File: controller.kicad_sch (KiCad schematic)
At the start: 6 parts, among them U1 ESP32-C6-DevKitC-1

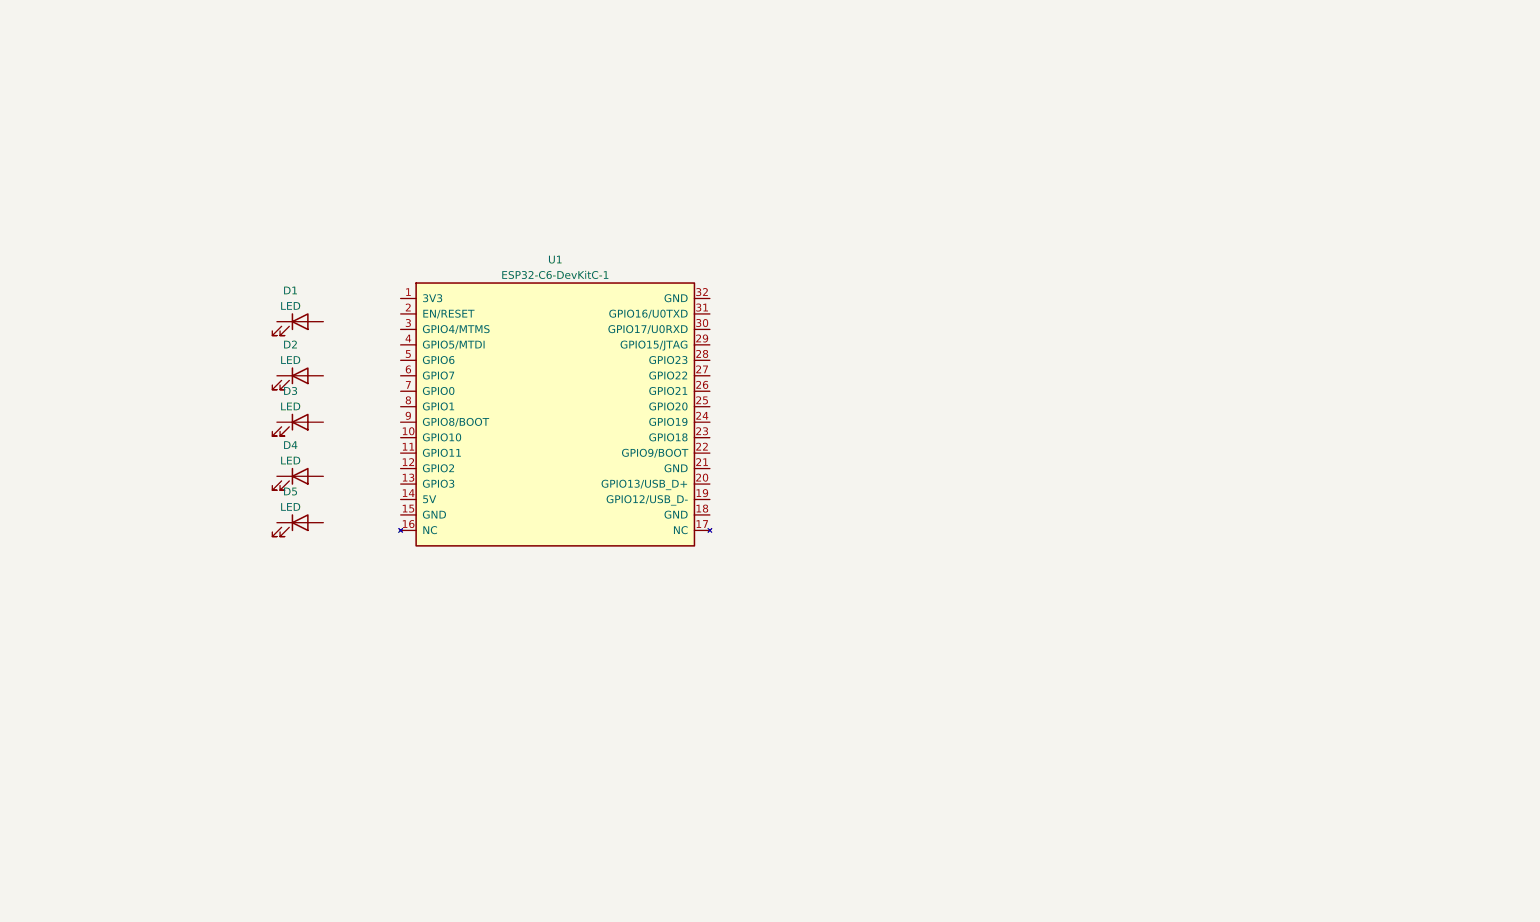
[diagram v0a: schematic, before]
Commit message: Initial routing
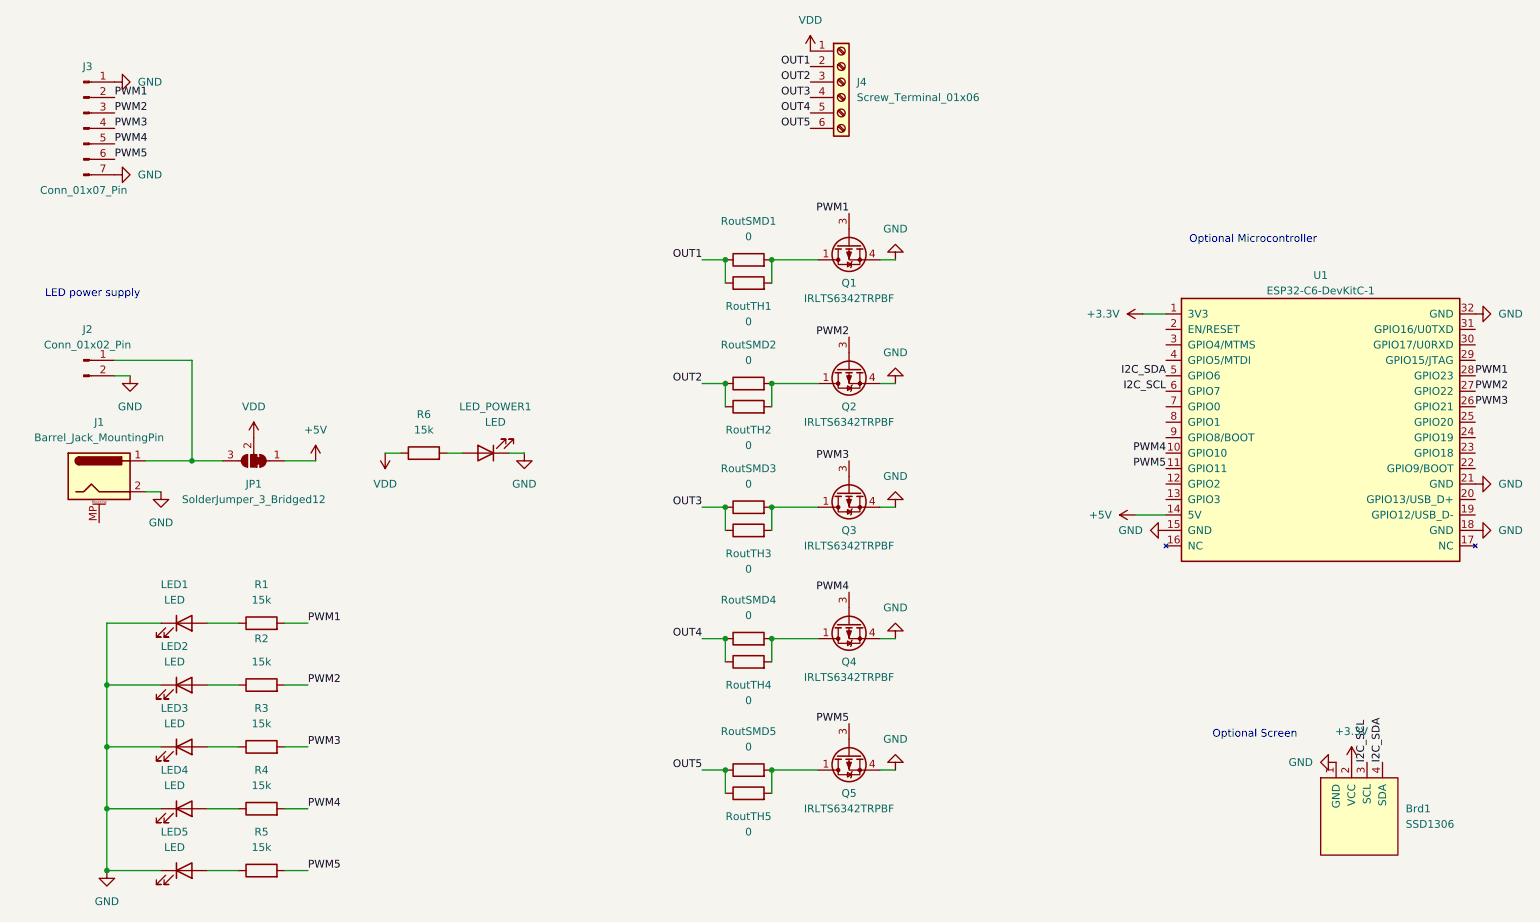
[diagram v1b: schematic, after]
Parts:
- added Brd1: SSD1306, SSD1306:128x64OLED, symbol SSD1306-128x64_OLED:SSD1306
- added J1: Barrel_Jack_MountingPin, Connector_BarrelJack:BarrelJack_CUI_PJ-063AH_Horizontal, symbol Connector:Barrel_Jack_MountingPin
- added J2: Conn_01x02_Pin, Connector_Molex:Molex_SL_171971-0002_1x02_P2.54mm_Vertical, symbol Connector:Conn_01x02_Pin
- added J3: Conn_01x07_Pin, Connector_Molex:Molex_SL_171971-0007_1x07_P2.54mm_Vertical, symbol Connector:Conn_01x07_Pin
- added J4: Screw_Terminal_01x06, TerminalBlock_RND:TerminalBlock_RND_205-00005_1x06_P5.00mm_Horizontal, symbol Connector:Screw_Terminal_01x06
- added JP1: SolderJumper_3_Bridged12, Jumper:SolderJumper-3_P1.3mm_Open_RoundedPad1.0x1.5mm_NumberLabels, symbol Jumper:SolderJumper_3_Bridged12
- added LED_POWER1: LED, LED_SMD:LED_0805_2012Metric_Pad1.15x1.40mm_HandSolder, symbol Device:LED
- added Q1, Q2, Q3, Q4, Q5: IRLTS6342TRPBF, Package_SO:TSOP-6_1.65x3.05mm_P0.95mm, symbol controller_library:IRLTS6342TRPBF
- added R1, R2, R3, R4, R5, R6: 15k, Resistor_SMD:R_0603_1608Metric_Pad0.98x0.95mm_HandSolder, symbol Device:R
- added RoutSMD1, RoutSMD2, RoutSMD3, RoutSMD4, RoutSMD5: 0, Resistor_SMD:R_0805_2012Metric_Pad1.20x1.40mm_HandSolder, symbol Device:R
- added RoutTH1, RoutTH2, RoutTH3, RoutTH4, RoutTH5: 0, Resistor_THT:R_Axial_DIN0204_L3.6mm_D1.6mm_P5.08mm_Horizontal, symbol Device:R
- LED1: renamed from D1; footprint (none) -> LED_SMD:LED_0805_2012Metric_Pad1.15x1.40mm_HandSolder
- LED2: renamed from D2; footprint (none) -> LED_SMD:LED_0805_2012Metric_Pad1.15x1.40mm_HandSolder
- LED3: renamed from D3; footprint (none) -> LED_SMD:LED_0805_2012Metric_Pad1.15x1.40mm_HandSolder
- LED4: renamed from D4; footprint (none) -> LED_SMD:LED_0805_2012Metric_Pad1.15x1.40mm_HandSolder
- LED5: renamed from D5; footprint (none) -> LED_SMD:LED_0805_2012Metric_Pad1.15x1.40mm_HandSolder
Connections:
- net +3.3V: now reaches U1.1 (3V3)
- net +3.3V: now also Brd1.2 (VCC)
- net PWM4: now reaches U1.10 (GPIO10)
- net PWM4: now also J3.5 (Pin_5), Q4.3 (G), R4.2
- net PWM5: now reaches U1.11 (GPIO11)
- net PWM5: now also J3.6 (Pin_6), Q5.3 (G), R5.2
- net +5V: now reaches U1.14 (5V)
- net +5V: now also JP1.1 (A)
- net GND: now reaches U1.15 (GND)
- net GND: now also LED1.1 (K), LED2.1 (K), LED3.1 (K), LED4.1 (K), LED5.1 (K), U1.18 (GND), U1.21 (GND), U1.32 (GND), Brd1.1 (GND), J1.2, J2.2 (Pin_2), J3.1 (Pin_1), J3.7 (Pin_7), LED_POWER1.1 (K), Q1.4 (S), Q2.4 (S), Q3.4 (S), Q4.4 (S), Q5.4 (S)
- net PWM3: now reaches U1.26 (GPIO21)
- net PWM3: now also J3.4 (Pin_4), Q3.3 (G), R3.2
- net PWM2: now reaches U1.27 (GPIO22)
- net PWM2: now also J3.3 (Pin_3), Q2.3 (G), R2.2
- net PWM1: now reaches U1.28 (GPIO23)
- net PWM1: now also J3.2 (Pin_2), Q1.3 (G), R1.2
- net I2C_SDA: now reaches U1.5 (GPIO6)
- net I2C_SDA: now also Brd1.4 (SDA)
- net I2C_SCL: now reaches U1.6 (GPIO7)
- net I2C_SCL: now also Brd1.3 (SCL)
- net at LED2.2 (A): now also R2.1
- net at LED1.2 (A): now also R1.1
- net at LED3.2 (A): now also R3.1
- net at LED4.2 (A): now also R4.1
- net at LED5.2 (A): now also R5.1
- new net: Q4.1 (D), Q4.2 (D), Q4.5 (D), Q4.6 (D), RoutSMD4.2, RoutTH4.2
- new net: Q3.1 (D), Q3.2 (D), Q3.5 (D), Q3.6 (D), RoutSMD3.2, RoutTH3.2
- new net: J1.1, J2.1 (Pin_1), JP1.3 (B)
- new net: Q1.1 (D), Q1.2 (D), Q1.5 (D), Q1.6 (D), RoutSMD1.2, RoutTH1.2
- new net: Q5.1 (D), Q5.2 (D), Q5.5 (D), Q5.6 (D), RoutSMD5.2, RoutTH5.2
- new net: Q2.1 (D), Q2.2 (D), Q2.5 (D), Q2.6 (D), RoutSMD2.2, RoutTH2.2
- new net: LED_POWER1.2 (A), R6.2
- new net OUT1: J4.2 (Pin_2), RoutSMD1.1, RoutTH1.1
- new net OUT2: J4.3 (Pin_3), RoutSMD2.1, RoutTH2.1
- new net OUT3: J4.4 (Pin_4), RoutSMD3.1, RoutTH3.1
- new net OUT4: J4.5 (Pin_5), RoutSMD4.1, RoutTH4.1
- new net OUT5: J4.6 (Pin_6), RoutSMD5.1, RoutTH5.1
- new net VDD: J4.1 (Pin_1), JP1.2 (C), R6.1
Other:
- note added: "LED power supply"
- note added: "Optional Microcontroller"
- note added: "Optional Screen"
- moved on the sheet: LED1, LED2, LED3, LED4, LED5, U1
